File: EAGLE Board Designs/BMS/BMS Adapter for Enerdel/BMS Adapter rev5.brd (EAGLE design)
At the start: 108 x 298.8 mm, 21 parts, among them X1 CONNECTOR-10, X2 CONNECTOR-10

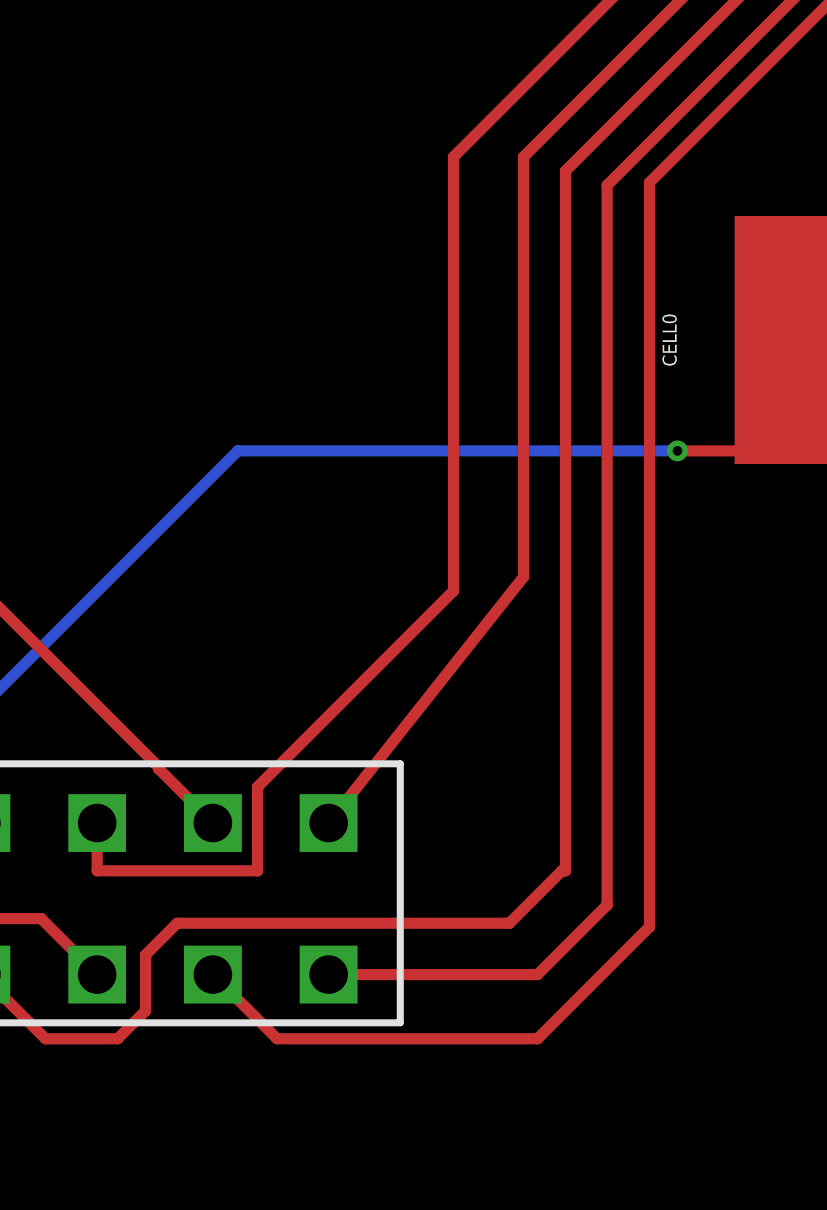
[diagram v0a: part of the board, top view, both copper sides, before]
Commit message: Update BMS Adapter rev5.brd
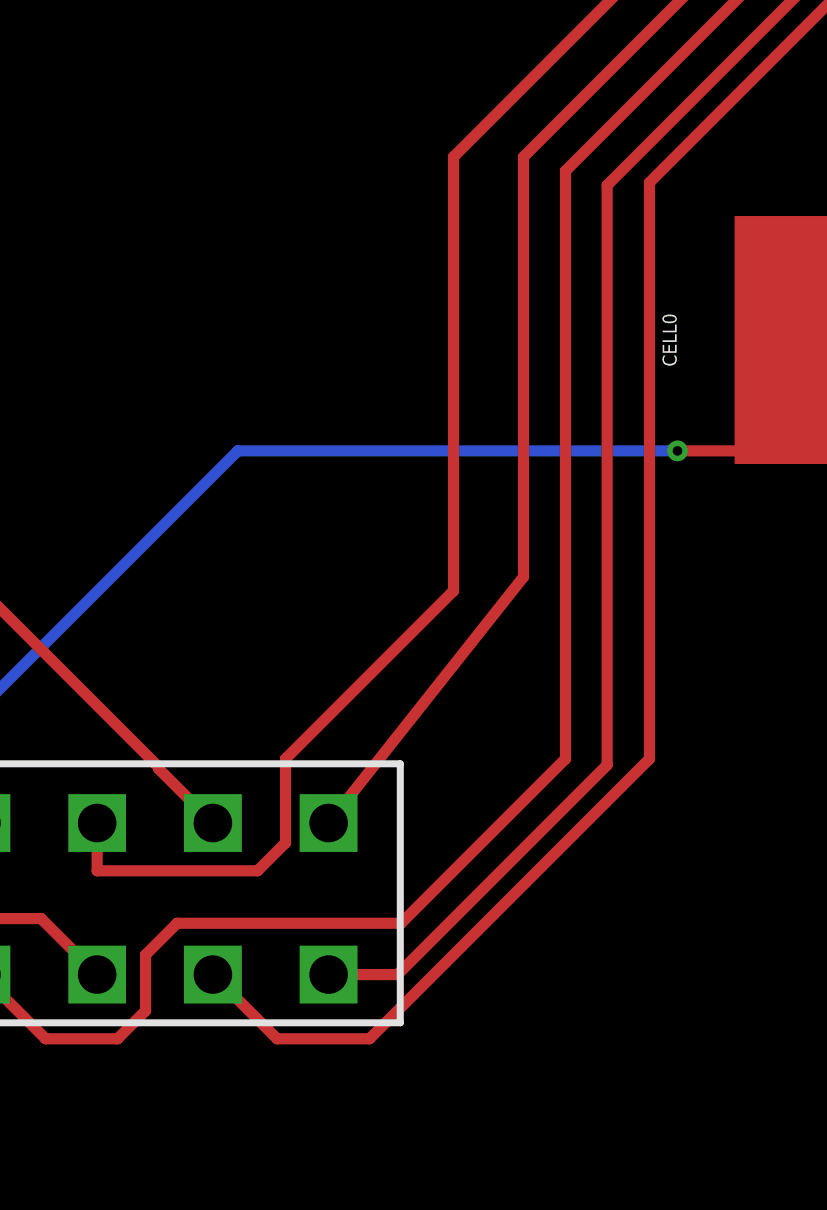
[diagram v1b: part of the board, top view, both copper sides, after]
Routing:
- net CELL8: track 160.0 -> 156.5 mm
- net CELL9: track 363.4 -> 360.4 mm
- net CELL6: track 138.5 -> 136.1 mm
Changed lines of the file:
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@@
 <wire x1="78.74" y1="29.464" x2="79" y2="29.89" width="0.4064" layer="1"/>
 <wire x1="48.027" y1="-12.49" x2="48.027" y2="-14.224" width="0.4064" layer="1"/>
-<wire x1="53.848" y1="-14.224" x2="53.848" y2="-11.176" width="0.4064" layer="1"/>
+<wire x1="54.864" y1="-13.208" x2="54.864" y2="-10.16" width="0.4064" layer="1"/>
 <wire x1="48.027" y1="-14.224" x2="53.848" y2="-14.224" width="0.4064" layer="1"/>
-<wire x1="53.848" y1="-11.176" x2="60.96" y2="-4.064" width="0.4064" layer="1"/>
+<wire x1="54.864" y1="-10.16" x2="60.96" y2="-4.064" width="0.4064" layer="1"/>
 <wire x1="60.96" y1="-4.064" x2="60.96" y2="11.684" width="0.4064" layer="1"/>
+<wire x1="53.848" y1="-14.224" x2="54.864" y2="-13.208" width="0.4064" layer="1"/>
 </signal>
 <signal name="CELL3">
@@
 <wire x1="79.248" y1="82.804" x2="85.344" y2="76.708" width="0.4064" layer="1"/>
 <wire x1="79.248" y1="82.804" x2="79" y2="83.19" width="0.4064" layer="1"/>
-<wire x1="65.024" y1="-14.224" x2="65.024" y2="11.176" width="0.4064" layer="1"/>
+<wire x1="65.024" y1="-10.16" x2="65.024" y2="11.176" width="0.4064" layer="1"/>
 <wire x1="65.024" y1="11.176" x2="76.2" y2="22.352" width="0.4064" layer="1"/>
 <wire x1="76.2" y1="22.352" x2="83.22484375" y2="22.352" width="0.4064" layer="1"/>
 <wire x1="85.25684375" y1="24.384" x2="85.344" y2="24.384" width="0.4064" layer="1"/>
 <wire x1="83.22484375" y1="22.352" x2="85.25684375" y2="24.384" width="0.4064" layer="1"/>
-<wire x1="62.992" y1="-16.1272" x2="64.8952" y2="-14.224" width="0.4064" layer="1"/>
-<wire x1="64.8952" y1="-14.224" x2="65.024" y2="-14.224" width="0.4064" layer="1"/>
+<wire x1="59.0568" y1="-16.1272" x2="65.024" y2="-10.16" width="0.4064" layer="1"/>
 <wire x1="43.827" y1="-17.99" x2="46.157" y2="-20.32" width="0.4064" layer="1"/>
 <wire x1="48.768" y1="-20.32" x2="49.784" y2="-19.304" width="0.4064" layer="1"/>
@@
 <wire x1="49.784" y1="-17.272" x2="50.9288" y2="-16.1272" width="0.4064" layer="1"/>
 <wire x1="46.157" y1="-20.32" x2="48.768" y2="-20.32" width="0.4064" layer="1"/>
-<wire x1="50.9288" y1="-16.1272" x2="62.992" y2="-16.1272" width="0.4064" layer="1"/>
+<wire x1="50.9288" y1="-16.1272" x2="59.0568" y2="-16.1272" width="0.4064" layer="1"/>
 </signal>
 <signal name="CELL7">
@@
 <wire x1="52.227" y1="-17.99" x2="54.557" y2="-20.32" width="0.4064" layer="1"/>
 <wire x1="79.248" y1="109.728" x2="79" y2="109.83" width="0.4064" layer="1"/>
-<wire x1="68.072" y1="-16.256" x2="68.072" y2="10.75515625" width="0.4064" layer="1"/>
+<wire x1="68.072" y1="-10.16" x2="68.072" y2="10.75515625" width="0.4064" layer="1"/>
 <wire x1="68.072" y1="10.75515625" x2="77.63684375" y2="20.32" width="0.4064" layer="1"/>
 <wire x1="77.63684375" y1="20.32" x2="84.328" y2="20.32" width="0.4064" layer="1"/>
 <wire x1="84.328" y1="20.32" x2="87.376" y2="23.368" width="0.4064" layer="1"/>
-<wire x1="54.557" y1="-20.32" x2="64.008" y2="-20.32" width="0.4064" layer="1"/>
-<wire x1="64.008" y1="-20.32" x2="68.072" y2="-16.256" width="0.4064" layer="1"/>
+<wire x1="54.557" y1="-20.32" x2="57.912" y2="-20.32" width="0.4064" layer="1"/>
+<wire x1="57.912" y1="-20.32" x2="68.072" y2="-10.16" width="0.4064" layer="1"/>
 </signal>
 <signal name="CELL9">
@@
 <wire x1="83.73284375" y1="21.336" x2="86.36" y2="23.96315625" width="0.4064" layer="1"/>
 <wire x1="77.216" y1="21.336" x2="83.73284375" y2="21.336" width="0.4064" layer="1"/>
-<wire x1="56.427" y1="-17.99" x2="64.008" y2="-17.99" width="0.4064" layer="1"/>
-<wire x1="64.008" y1="-17.99" x2="66.535" y2="-15.463" width="0.4064" layer="1"/>
-<wire x1="66.535" y1="-15.463" x2="66.535" y2="10.655" width="0.4064" layer="1"/>
+<wire x1="56.427" y1="-17.99" x2="58.928" y2="-17.99" width="0.4064" layer="1"/>
+<wire x1="58.928" y1="-17.99" x2="66.535" y2="-10.383" width="0.4064" layer="1"/>
+<wire x1="66.535" y1="-10.383" x2="66.535" y2="10.655" width="0.4064" layer="1"/>
 </signal>
 <signal name="CELL10">
